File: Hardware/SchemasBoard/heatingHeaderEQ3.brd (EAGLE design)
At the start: 45.5 x 30.5 mm, 36 parts, among them IC1 DS1820, T5 BC846

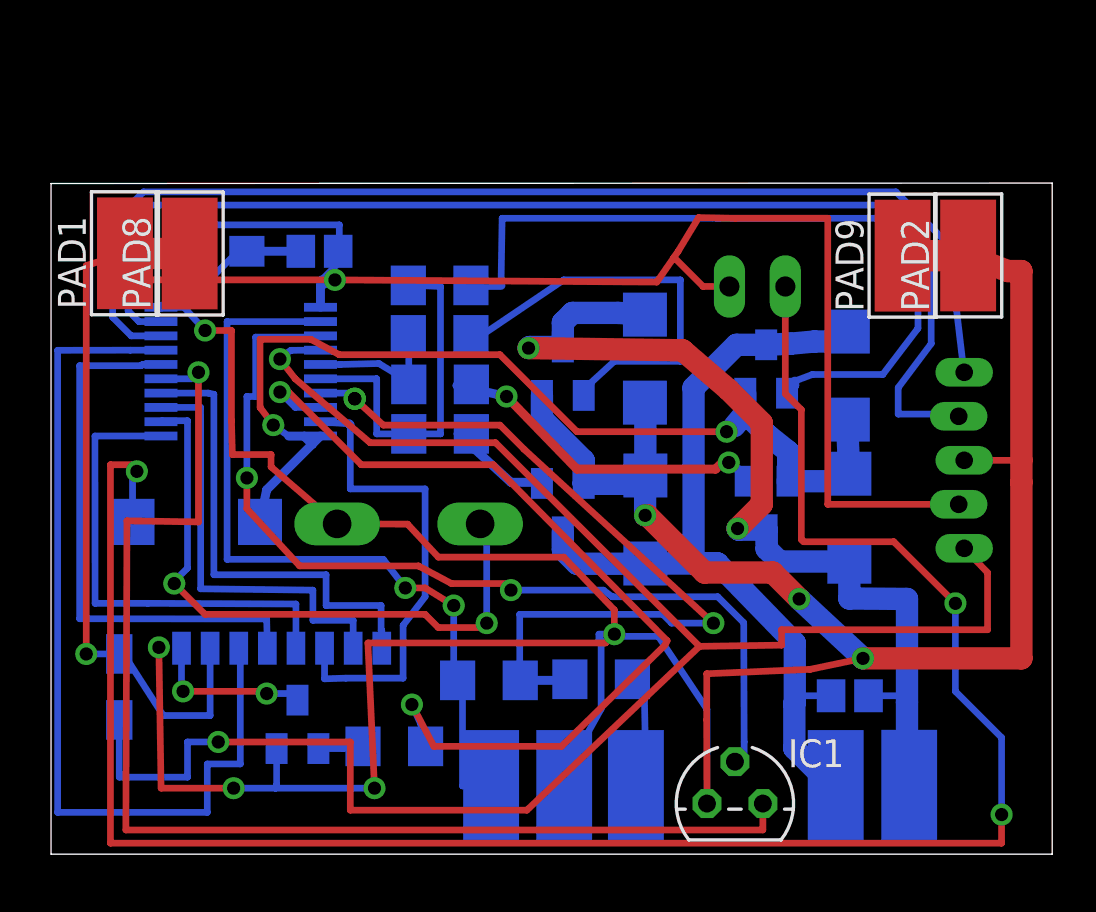
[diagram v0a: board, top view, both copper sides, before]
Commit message: a
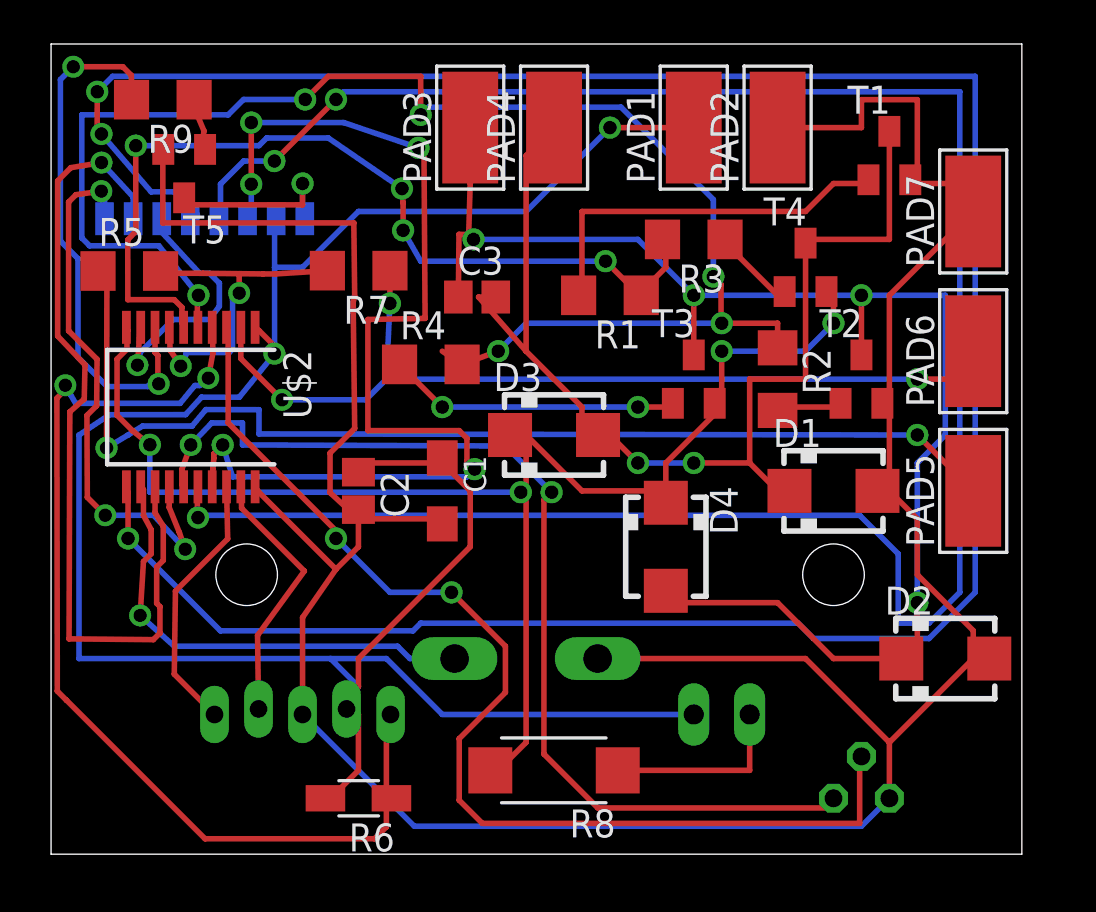
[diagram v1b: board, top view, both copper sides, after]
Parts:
- removed PAD8, PAD9: WIREPADSMD5-2,5, wirepad:5-2,5
- moved U$1 48.4 mm to (11.4, 43.2), turned to 0 degrees
- moved PAD3 36.0 mm to (19.1, 33.0), flipped to the top
- moved PAD4 32.5 mm to (22.9, 33.0), flipped to the top
- moved U$3 32.2 mm to (11.4, 6.35), flipped to the bottom, turned to 0 degrees
- moved PAD7 32.1 mm to (41.9, 29.2), flipped to the top
- moved R9 31.2 mm to (5.08, 34.3), flipped to the top
- moved PAD6 29.5 mm to (41.9, 22.9), flipped to the top
- moved R5 28.4 mm to (3.56, 26.5), flipped to the top
- moved PAD1 26.5 mm to (29.2, 33.0)
- moved T5 25.6 mm to (6.05, 30.9), flipped to the top, turned to 180 degrees
- moved C3 24.8 mm to (19.4, 25.3), flipped to the top
- moved T1 21.8 mm to (38.1, 31.8), flipped to the top, turned to 0 degrees
- moved PAD5 20.4 mm to (41.9, 16.5), flipped to the top
- moved R8 19.8 mm to (22.9, 3.81), flipped to the top
- moved R7 19.5 mm to (14.0, 26.5), flipped to the top
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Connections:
- net GND: no longer PAD9.1
- net VDD: no longer PAD8.1
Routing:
- net N$22: track 21.7 -> 115.9 mm, vias 0 -> 3
- net N$2: track 93.5 -> 8.53 mm, vias 3 -> 0
- net N$20: track 25.0 -> 100.2 mm, vias 0 -> 3
- net N$31: track 6.60 -> 69.8 mm, vias 0 -> 6
- net N$4: track 5.45 -> 50.6 mm, vias 0 -> 2
- net N$18: track 54.7 -> 12.0 mm
- net N$19: track 53.1 -> 12.1 mm
- net GND: track 172.3 -> 138.8 mm, vias 8 -> 0
- net N$25: track 81.0 -> 47.5 mm
- net N$27: track 34.7 -> 4.11 mm
- net N$30: track 16.1 -> 41.2 mm, vias 0 -> 4
- net N$7: track 44.6 -> 66.4 mm, vias 2 -> 4
- net N$12: track 36.5 -> 16.2 mm
- net N$15: track 46.2 -> 65.4 mm, vias 2 -> 4
- net N$6: track 19.6 -> 38.2 mm, vias 0 -> 1
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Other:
- board size 45.5 x 30.5 mm -> 44.1 x 36.8 mm
